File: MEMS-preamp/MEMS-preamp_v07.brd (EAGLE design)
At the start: 50 x 30.1 mm, 45 parts, among them IC1 DMN2400, IC2 BQ21040, IC3 BQ297X, IC4 SC4503, IC5 TPS7A49, IC6 OPA2134, J2 Battery, SW1 SPDT

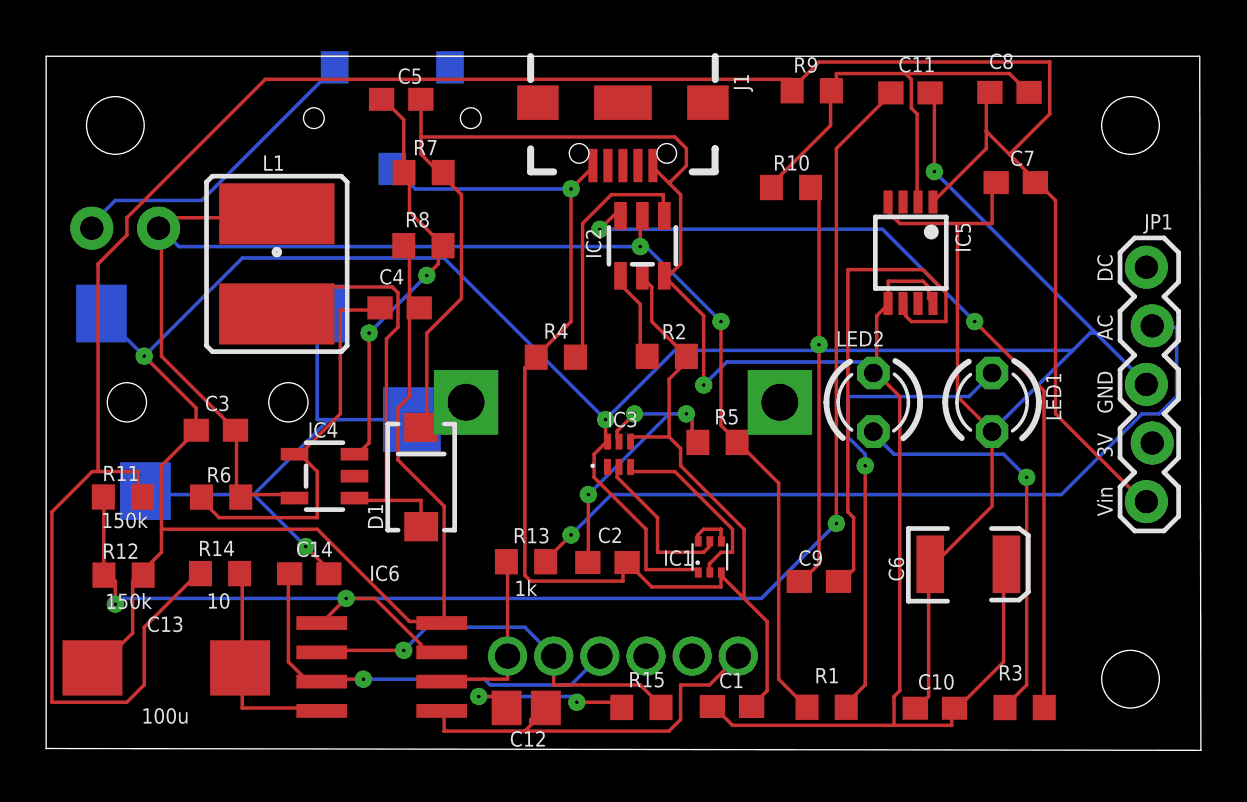
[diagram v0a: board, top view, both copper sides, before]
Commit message: boards layed out
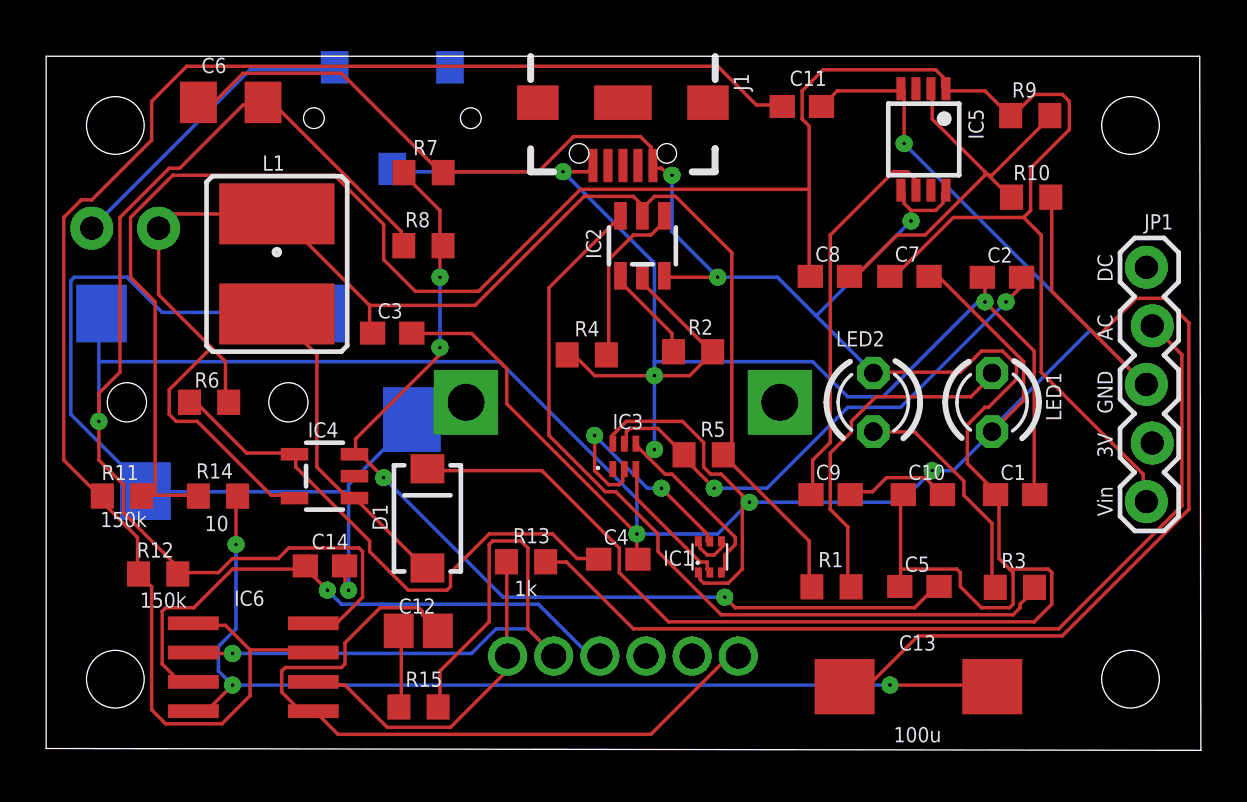
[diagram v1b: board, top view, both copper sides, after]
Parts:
- C1, C10, C2, C3, C7, C8: device adafruit:C0603 -> rcl:C0603
- C4: value 56nf -> 56nF; device adafruit:C0603 -> rcl:C0603
- C5: value 2.2pf -> 2.2pF; device adafruit:C0603 -> rcl:C0603
- C6: device SparkFun:EIA3528 -> rcl:C1206
- C9: value 10nF -> 10uF; device adafruit:C0603 -> rcl:C0603
- moved C6 37.7 mm to (8.00, 28.0)
- moved C13 32.6 mm to (37.8, 2.68)
- moved C5 30.8 mm to (37.9, 7.02), turned to 0 degrees
- moved C2 21.1 mm to (41.4, 20.4)
- moved C1 15.3 mm to (42.0, 11.0)
- moved C4 14.4 mm to (24.8, 8.20)
- moved C8 11.1 mm to (34.0, 20.5)
- moved R10 10.4 mm to (42.7, 23.9)
- moved R15 9.66 mm to (16.1, 1.79)
- moved R9 9.53 mm to (42.7, 27.4)
- moved C10 9.27 mm to (38.0, 11.0), turned to 0 degrees
- moved C3 8.73 mm to (15.0, 18.0), turned to 0 degrees
- moved C7 6.14 mm to (37.4, 20.5), turned to 0 degrees
- moved C12 5.75 mm to (16.1, 5.09)
- moved IC6 5.56 mm to (8.98, 3.52)
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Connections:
- net GND: now also C6.2; no longer C6.C
- net GND2: now also C2.1; no longer C2.2
- net N$18: now also C2.2; no longer C2.1
- net V+: now also C6.1; no longer C6.A
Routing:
- net N$1: track 9.46 -> 43.9 mm, vias 0 -> 3
- net GND: track 178.1 -> 209.5 mm, vias 4 -> 5
- net N$14: track 18.3 -> 43.0 mm, vias 2 -> 4
- net V+: track 90.0 -> 113.3 mm, vias 1 -> 3
- net N$7: track 22.8 -> 40.2 mm
- net N$9: track 17.4 -> 31.8 mm
- net GROU[: track 17.4 -> 31.6 mm
- net N$18: track 13.1 -> 23.0 mm, vias 3 -> 2
- net +12V: track 108.6 -> 99.0 mm
- net N$11: track 17.9 -> 10.0 mm, vias 1 -> 0
- net N$8: track 64.1 -> 71.5 mm, vias 3 -> 0
- net N$10: track 18.4 -> 25.4 mm
- net N$5: track 8.00 -> 15.0 mm
- net GND2: track 62.7 -> 69.5 mm, vias 1 -> 4
- net N$13: track 17.5 -> 23.5 mm
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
